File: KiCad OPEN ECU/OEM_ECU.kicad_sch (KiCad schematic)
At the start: 46 parts, among them J1 TYPE-C-31-M-12, J6 RFShield_OnePiece, U1 ATSHA204A-MAHDA-T, U1 ESP32C3

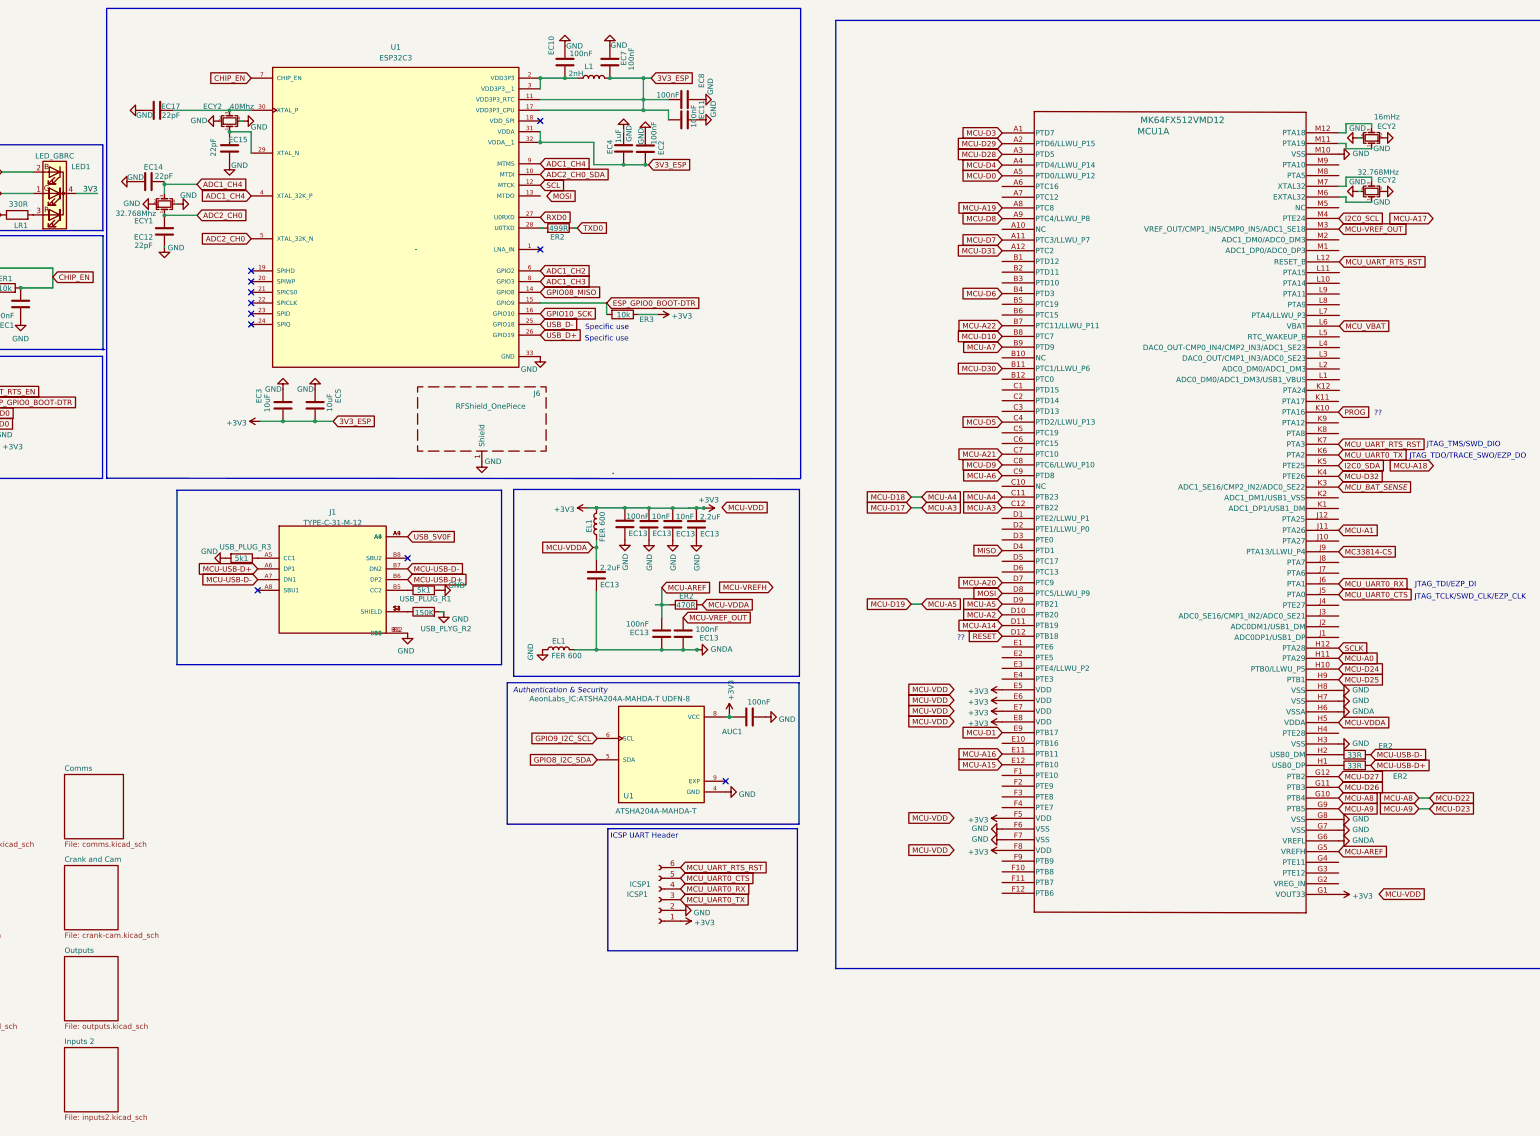
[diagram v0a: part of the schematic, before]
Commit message: Add files via upload
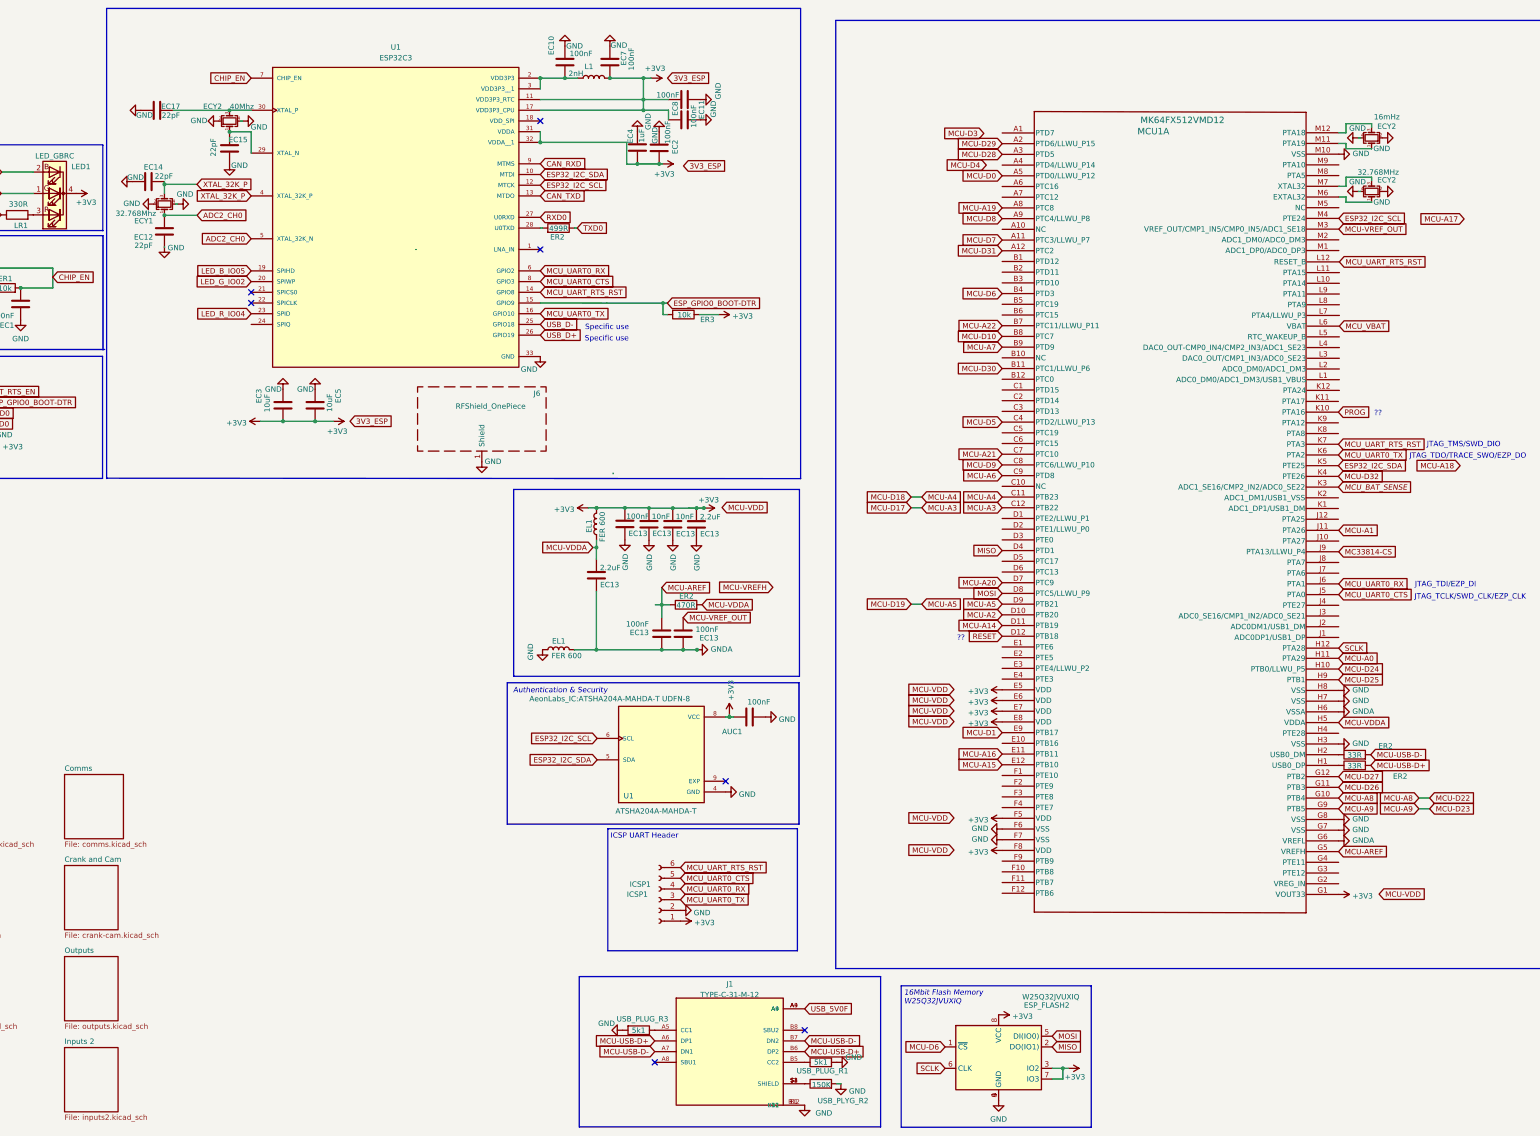
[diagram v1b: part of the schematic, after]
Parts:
- added ESP_FLASH2: W25Q32JVUXIQ, AeonLabs_IC:WSON8 FLASH SPI SON127P800X600X80-9N, symbol Memory_Flash:SPI_Flash_W25Q128JVS
- LED1: footprint LED_SMD:LED_1206_3210_RGB_Metric -> AeonLabs_Power:LED_1206_3210_RGB_Metric
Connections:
- net 3V3 is gone; now on net +3V3: LED1.4 (K)
- net ADC1_CH2 is gone; now on net MCU_UART0_RX: U1.6 (GPIO2)
- net ADC1_CH3 is gone; now on net MCU_UART0_CTS: U1.8 (GPIO3)
- net GPIO08_MISO is gone; now on net MCU_UART_RTS_RST: U1.14 (GPIO8)
- net GPIO10_SCK is gone; now on net MCU_UART0_TX: U1.16 (GPIO10)
- net GPIO8_I2C_SDA is gone; now on net ESP32_I2C_SDA: U1.5 (SDA)
- net I2C0_SCL is gone; now on net ESP32_I2C_SCL: MCU1.M4 (PTE24)
- net I2C0_SDA is gone; now on net ESP32_I2C_SDA: MCU1.K5 (PTE25)
- net SCL is gone; now on net ESP32_I2C_SCL: U1.12 (MTCK)
- net +3V3: now also ESP_FLASH2.3 (IO2), ESP_FLASH2.7 (IO3), ESP_FLASH2.8 (VCC)
- net GND: now also ESP_FLASH2.4 (GND), ESP_FLASH2.9 (GND)
- net LED_B_IO05: now also U1.19 (SPIHD)
- net LED_G_IO02: now also U1.20 (SPIWP)
- net LED_R_IO04: now also U1.23 (SPID)
- net MCU-D3: no longer MCU1.A1 (PTD7)
- net MCU-D4: no longer MCU1.A4 (PTD4/LLWU_P14)
- net MCU-D6: now also ESP_FLASH2.1 (~{CS})
- net MISO: now also ESP_FLASH2.2 (DO(IO1))
- net MOSI: now also ESP_FLASH2.5 (DI(IO0))
- net SCLK: now also ESP_FLASH2.6 (CLK)
- net CAN_TXD: now reaches U1.13 (MTDO)
- net ADC1_CH4 renamed XTAL_32K_P
- net XTAL_32K_P: no longer U1.9 (MTMS)
- net ADC2_CH0_SDA renamed ESP32_I2C_SDA
- net GPIO9_I2C_SCL renamed ESP32_I2C_SCL
- new net CAN_RXD: U1.9 (MTMS)
- no-connect marks 11 -> 7
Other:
- note added: "16Mbit Flash Memory W25Q32JVUXIQ"
- moved on the sheet: EC2, EC4, ER3, J1, USB_PLUG_R1, USB_PLUG_R3, USB_PLYG_R2
